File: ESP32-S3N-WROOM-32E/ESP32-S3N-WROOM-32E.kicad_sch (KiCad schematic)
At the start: 51 parts, among them J1 Conn_01x19_Socket, J10 Conn_01x22_Socket, J16 XT60-M, J17 XT60-M, J2 Conn_01x19_Socket, J3 Conn_01x19_Socket, J4 Conn_01x19_Socket, J5 Conn_01x02_Pin, J6 Conn_01x02_Pin, J7 Conn_01x22_Socket, J8 Conn_01x22_Socket, J9 Conn_01x22_Socket, SW1 SW1, SW2 SW2, SW3 SW3, SW4 SW4, SW5 SW5, SW6 SW6, SW7 SW7, SW8 SW7

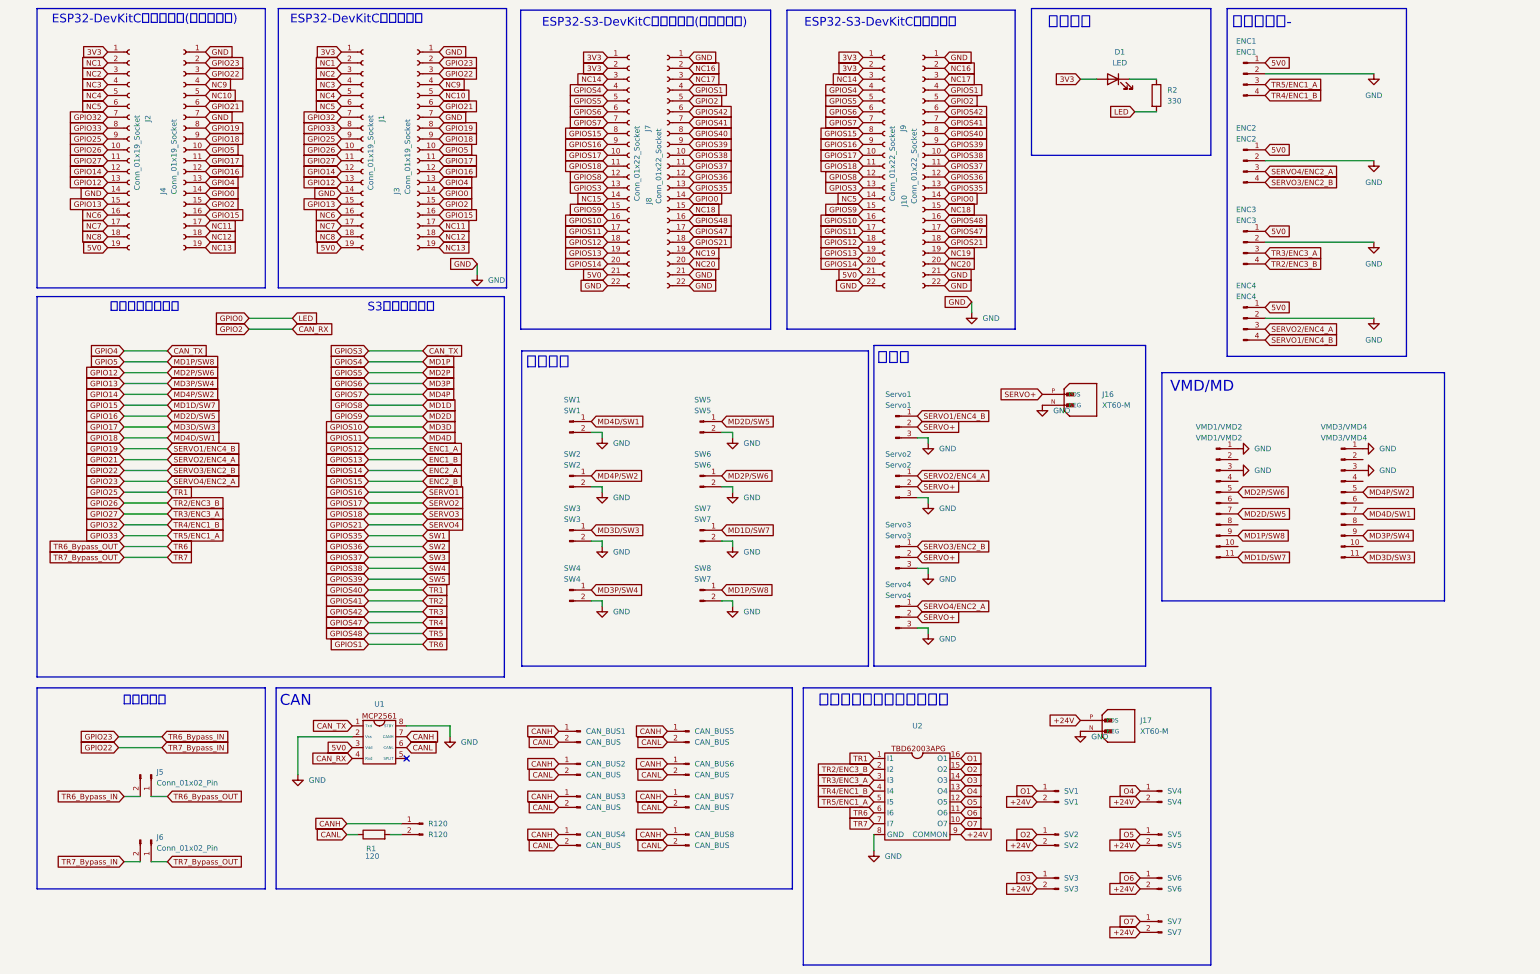
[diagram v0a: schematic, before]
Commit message: 回路図２
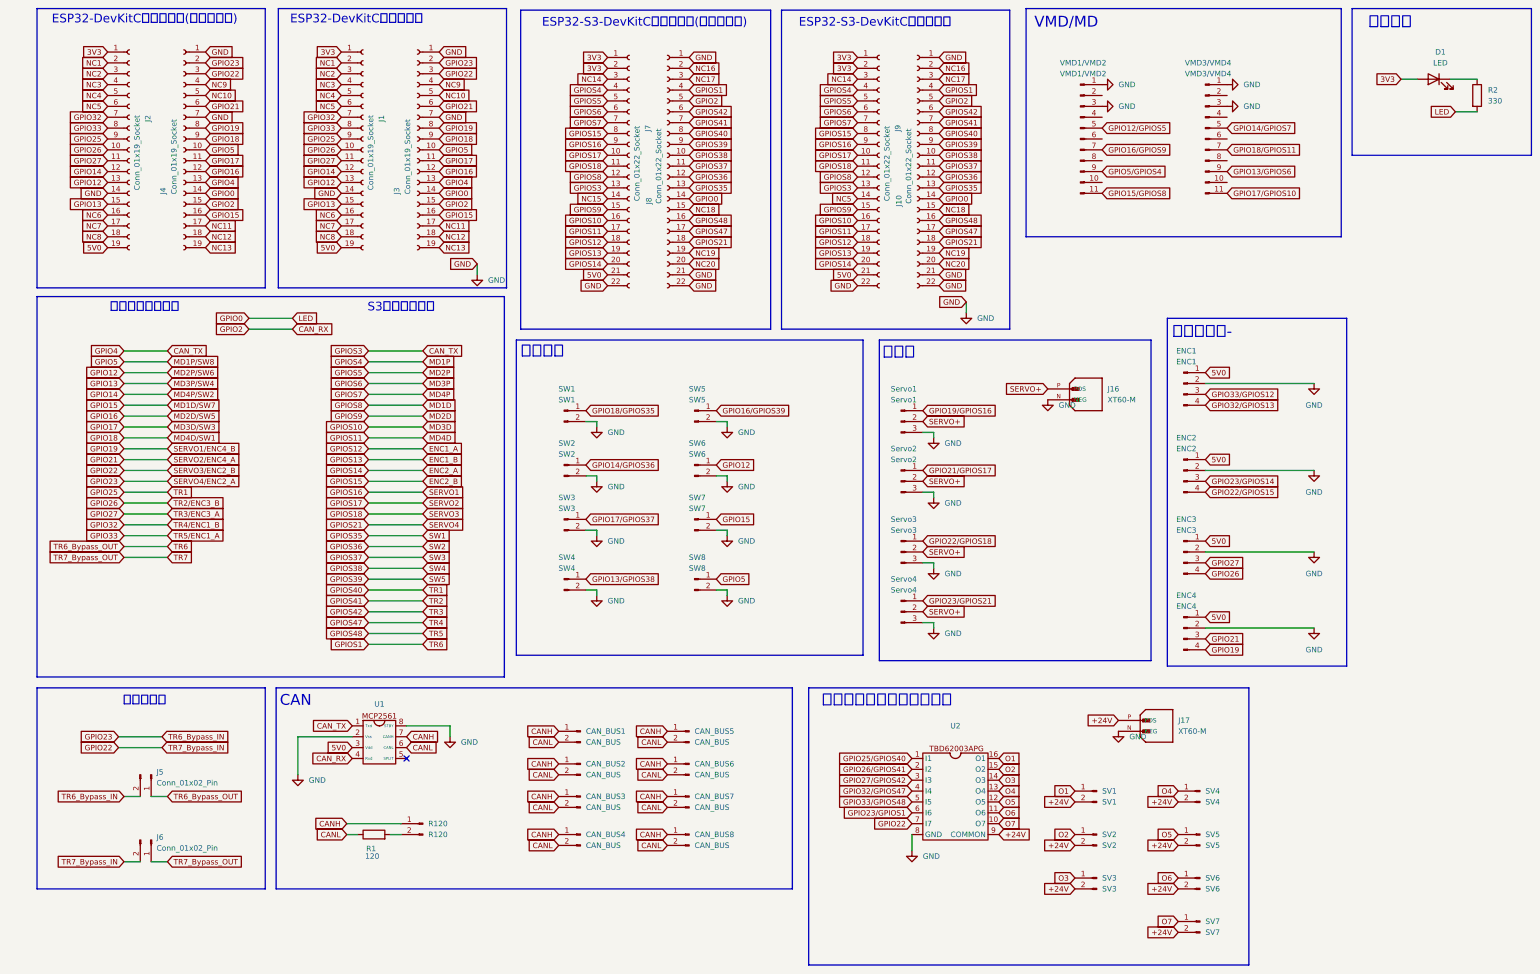
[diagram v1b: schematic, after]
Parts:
- SW8: value SW7 -> SW8
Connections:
- net GPIO12: no longer VMD1/VMD2.5 (Pin_5)
- net GPIO13: no longer SW4.1 (Pin_1), VMD3/VMD4.9 (Pin_9)
- net GPIO14: no longer SW2.1 (Pin_1), VMD3/VMD4.5 (Pin_5)
- net GPIO15: no longer VMD1/VMD2.11 (Pin_11)
- net GPIO16: no longer SW5.1 (Pin_1), VMD1/VMD2.7 (Pin_7)
- net GPIO17: no longer SW3.1 (Pin_1), VMD3/VMD4.11 (Pin_11)
- net GPIO18: no longer SW1.1 (Pin_1), VMD3/VMD4.7 (Pin_7)
- net GPIO19: no longer Servo1.1 (Pin_1)
- net GPIO21: no longer Servo2.1 (Pin_1)
- net GPIO22: now also U2.7 (I7); no longer ENC2.4 (Pin_4), Servo3.1 (Pin_1)
- net GPIO23: no longer ENC2.3 (Pin_3), Servo4.1 (Pin_1)
- net GPIO25: no longer U2.1 (I1)
- net GPIO26: no longer U2.2 (I2)
- net GPIO27: no longer U2.3 (I3)
- net GPIO32: no longer ENC1.4 (Pin_4), U2.4 (I4)
- net GPIO33: no longer ENC1.3 (Pin_3), U2.5 (I5)
- net GPIO5: no longer VMD1/VMD2.9 (Pin_9)
- net GPIOS1: no longer U2.6 (I6)
- net TR7: no longer U2.7 (I7)
- new net GPIO12/GPIOS5: VMD1/VMD2.5 (Pin_5)
- new net GPIO13/GPIOS38: SW4.1 (Pin_1)
- new net GPIO13/GPIOS6: VMD3/VMD4.9 (Pin_9)
- new net GPIO14/GPIOS36: SW2.1 (Pin_1)
- new net GPIO14/GPIOS7: VMD3/VMD4.5 (Pin_5)
- new net GPIO15/GPIOS8: VMD1/VMD2.11 (Pin_11)
- new net GPIO16/GPIOS39: SW5.1 (Pin_1)
- new net GPIO16/GPIOS9: VMD1/VMD2.7 (Pin_7)
- new net GPIO17/GPIOS10: VMD3/VMD4.11 (Pin_11)
- new net GPIO17/GPIOS37: SW3.1 (Pin_1)
- new net GPIO18/GPIOS11: VMD3/VMD4.7 (Pin_7)
- new net GPIO18/GPIOS35: SW1.1 (Pin_1)
- new net GPIO19/GPIOS16: Servo1.1 (Pin_1)
- new net GPIO21/GPIOS17: Servo2.1 (Pin_1)
- new net GPIO22/GPIOS15: ENC2.4 (Pin_4)
- new net GPIO22/GPIOS18: Servo3.1 (Pin_1)
- new net GPIO23/GPIOS1: U2.6 (I6)
- new net GPIO23/GPIOS14: ENC2.3 (Pin_3)
- new net GPIO23/GPIOS21: Servo4.1 (Pin_1)
- new net GPIO25/GPIOS40: U2.1 (I1)
- new net GPIO26/GPIOS41: U2.2 (I2)
- new net GPIO27/GPIOS42: U2.3 (I3)
- new net GPIO32/GPIOS13: ENC1.4 (Pin_4)
- new net GPIO32/GPIOS47: U2.4 (I4)
- new net GPIO33/GPIOS12: ENC1.3 (Pin_3)
- new net GPIO33/GPIOS48: U2.5 (I5)
- new net GPIO5/GPIOS4: VMD1/VMD2.9 (Pin_9)
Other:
- moved on the sheet: D1, ENC1, ENC2, ENC3, ENC4, J10, J16, J17, J9, R2, SV1, SV2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
